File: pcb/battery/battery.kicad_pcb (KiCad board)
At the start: 2 copper layers, 147 parts, among them J1 Conn_01x11_Pin, J2 p2.0, J3 p2.0, J4 UART XH2.54, J5 p2.0, J6 P+/C+, J7 PN/CN, J8 B+, J9 B-, Q1 MMBT5401, Q2 BSC030N08NS5, Q3 BSC030N08NS5, Q4 BSC030N08NS5, Q5 BSC030N08NS5, U1 SH3676010B, U10 ETA3000_DFN2x2, U2 ETA3000_DFN2x2, U3 ETA3000_DFN2x2, U4 ETA3000_DFN2x2, U5 ETA3000_DFN2x2, U6 ETA3000_DFN2x2, U7 ETA3000_DFN2x2, U8 ETA3000_DFN2x2, U9 ETA3000_DFN2x2

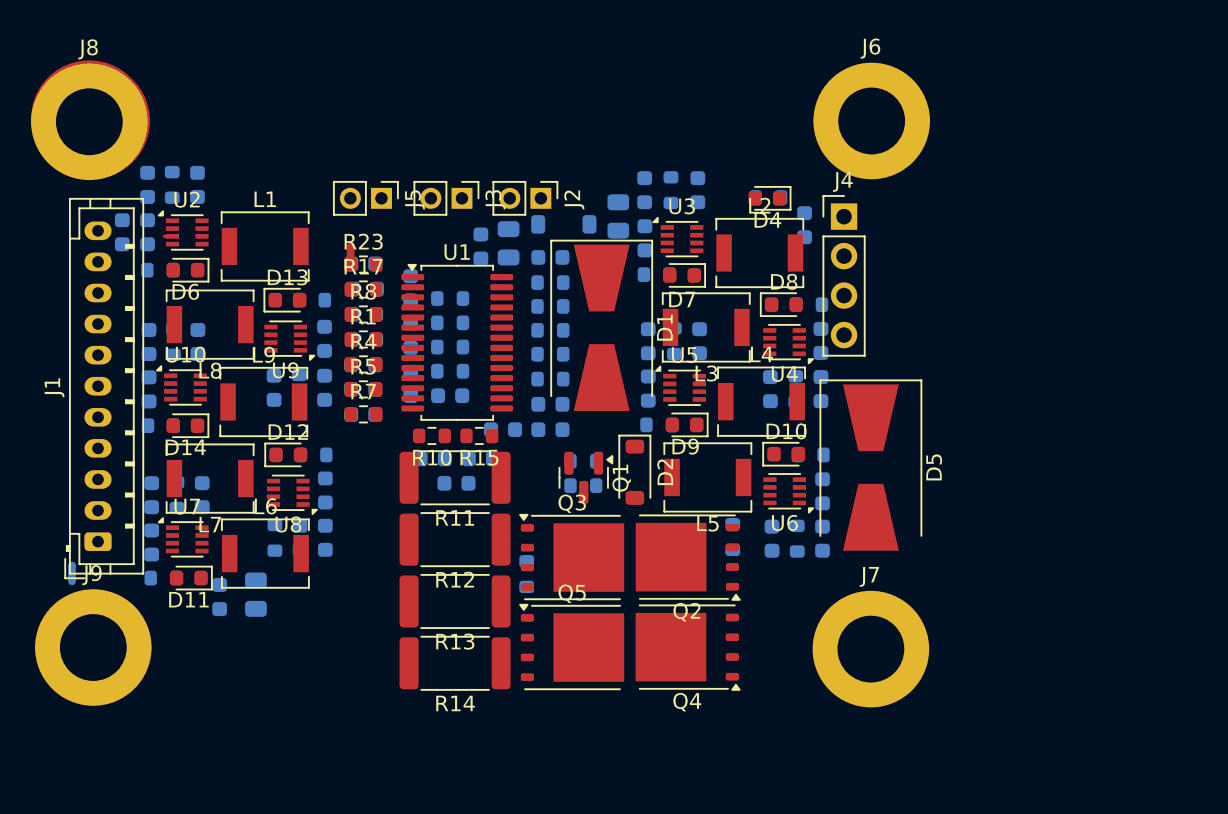
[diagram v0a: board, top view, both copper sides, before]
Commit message: feat: update
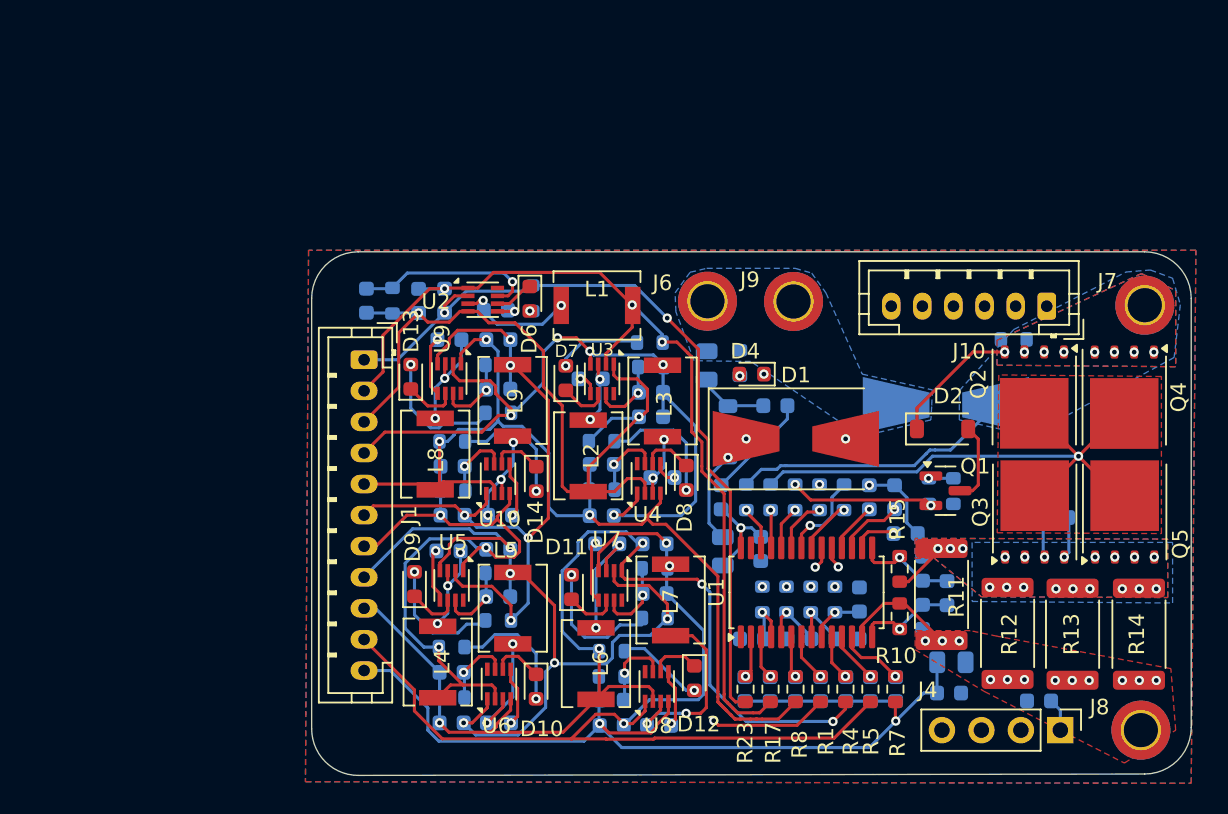
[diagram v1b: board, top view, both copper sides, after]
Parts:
- removed J2, J3, J5: p2.0, Connector_PinHeader_2.00mm:PinHeader_1x02_P2.00mm_Vertical
- removed NT1: power, NetTie:NetTie-2_SMD_Pad0.5mm
- removed NT3: sensor, NetTie:NetTie-2_SMD_Pad0.5mm
- added J10: Conn_01x06_Pin, Connector_JST:JST_PH_B6B-PH-K_1x06_P2.00mm_Vertical, F.Cu at (181.9, 95.4)
- D5: moved to B.Cu
- J6, J7: footprint MountingHole:MountingHole_4.3mm_M4_DIN965_Pad -> MountingHole:MountingHole_2.2mm_M2_DIN965_Pad_TopBottom
- J8: value B+ -> PN/CN; footprint MountingHole:MountingHole_4.3mm_M4_DIN965_Pad -> MountingHole:MountingHole_2.2mm_M2_DIN965_Pad_TopBottom
- J9: value B- -> P+/C+; footprint MountingHole:MountingHole_4.3mm_M4_DIN965_Pad -> MountingHole:MountingHole_2.2mm_M2_DIN965_Pad_TopBottom
- moved J8 78.2 mm to (188.0, 122.7)
- moved J9 50.3 mm to (165.6, 95.1)
- moved C2 47.3 mm to (175.6, 120.3), turned to 180 degrees
- moved R2 45.0 mm to (175.8, 118.3), turned to 180 degrees
- moved R14 44.0 mm to (187.8, 116.5), turned to -90 degrees
- moved R13 39.8 mm to (183.6, 116.5), turned to -90 degrees
- moved C8 38.5 mm to (172.2, 120.0), turned to 90 degrees
- moved R7 38.5 mm to (172.2, 120.0), turned to 90 degrees
- moved C5 37.9 mm to (170.6, 120.0), turned to 90 degrees
- moved R5 37.9 mm to (170.6, 120.0), turned to 90 degrees
- moved C4 37.4 mm to (169.0, 120.0), turned to 90 degrees
- moved R4 37.4 mm to (168.9, 120.0), turned to 90 degrees
- moved R1 37.0 mm to (167.3, 120.0), turned to 90 degrees
- moved C1 37.0 mm to (167.4, 120.0), turned to 90 degrees
- moved R8 36.8 mm to (165.7, 120.0), turned to 90 degrees
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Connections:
- C2 pad 1: B- -> GND
- J8 pad 1: B+/P+/C+ -> GND
- J9 pad 1: B- -> B+/P+/C+
- R10 pad 1: B- -> GND
- R11 pad 2: B- -> GND
- R12 pad 2: B- -> GND
- R13 pad 2: B- -> GND
- R14 pad 2: B- -> GND
- R2 pad 1: B- -> GND
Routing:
- net /B8: track 0.00 -> 72.5 mm, vias 0 -> 3
- net /B5: track 0.00 -> 71.1 mm, vias 0 -> 6
- net /B2: track 0.00 -> 70.9 mm, vias 0 -> 5
- net /B3: track 0.00 -> 67.1 mm, vias 0 -> 6
- net /B1: track 0.00 -> 66.6 mm, vias 0 -> 3
- net /B4: track 0.00 -> 66.2 mm, vias 0 -> 4
- net /B6: track 0.00 -> 65.1 mm, vias 0 -> 3
- net /B7: track 0.00 -> 63.2 mm, vias 0 -> 6
- net /B9: track 0.06 -> 61.0 mm, vias 0 -> 3
- net /B0: track 0.00 -> 54.6 mm, vias 0 -> 2
- net /B10: track 0.00 -> 51.7 mm, vias 0 -> 2
- net Net-(Q2-D): track 0.00 -> 36.5 mm, vias 0 -> 1
- net GND: track 0.00 -> 29.6 mm, vias 0 -> 15
- net +5V: track 0.00 -> 28.6 mm, vias 0 -> 1
- net Net-(Q3-G): track 0.00 -> 28.0 mm, vias 0 -> 3
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- added copper zone on B.Cu, net B+/P+/C+
- added copper zone on B.Cu, net GND
- added copper zone on F.Cu, net GND
- added copper zone on In1.Cu, net GND
- added copper zone on In2.Cu, net GND
- added copper zone on In3.Cu, net GND
- added copper zone on In4.Cu, net GND
- added copper zone on F.Cu, net Net-(Q2-D)
- added copper zone on B.Cu, net Net-(Q3-S-Pad1)
- added copper zone on F.Cu, net Net-(Q3-S-Pad1)
- added copper zone on In1.Cu, net Net-(Q3-S-Pad1)
- added copper zone on In2.Cu, net Net-(Q3-S-Pad1)
- added copper zone on In3.Cu, net Net-(Q3-S-Pad1)
- added copper zone on In4.Cu, net Net-(Q3-S-Pad1)
- added copper zone on B.Cu, net PN/CN
- added copper zone on F.Cu, net PN/CN
- added copper zone on In1.Cu, net PN/CN
- added copper zone on In2.Cu, net PN/CN
- added copper zone on In3.Cu, net PN/CN
- added copper zone on In4.Cu, net PN/CN
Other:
- board outline added: 56.6 x 33.7 mm
- copper layers 2 -> 6
